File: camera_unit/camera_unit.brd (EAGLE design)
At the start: 87 x 50 mm, 0 parts

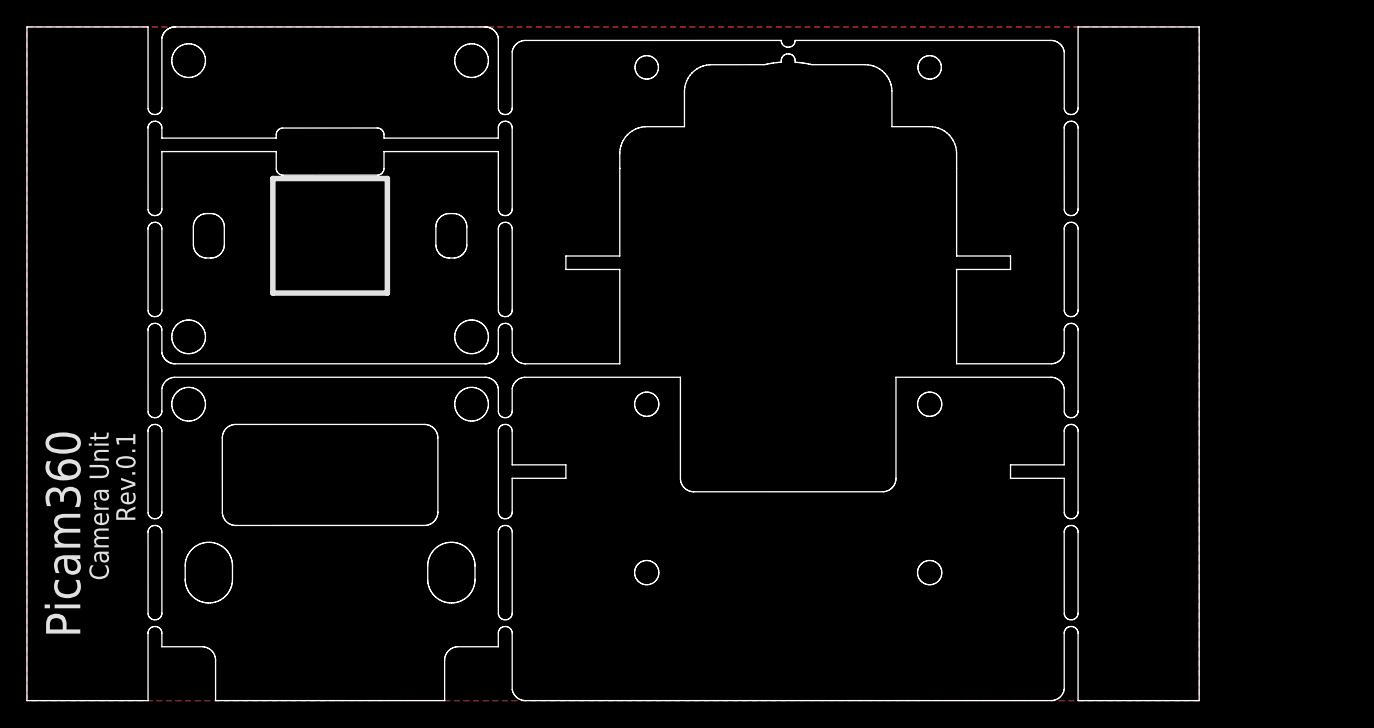
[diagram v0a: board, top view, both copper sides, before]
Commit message: before autorouter
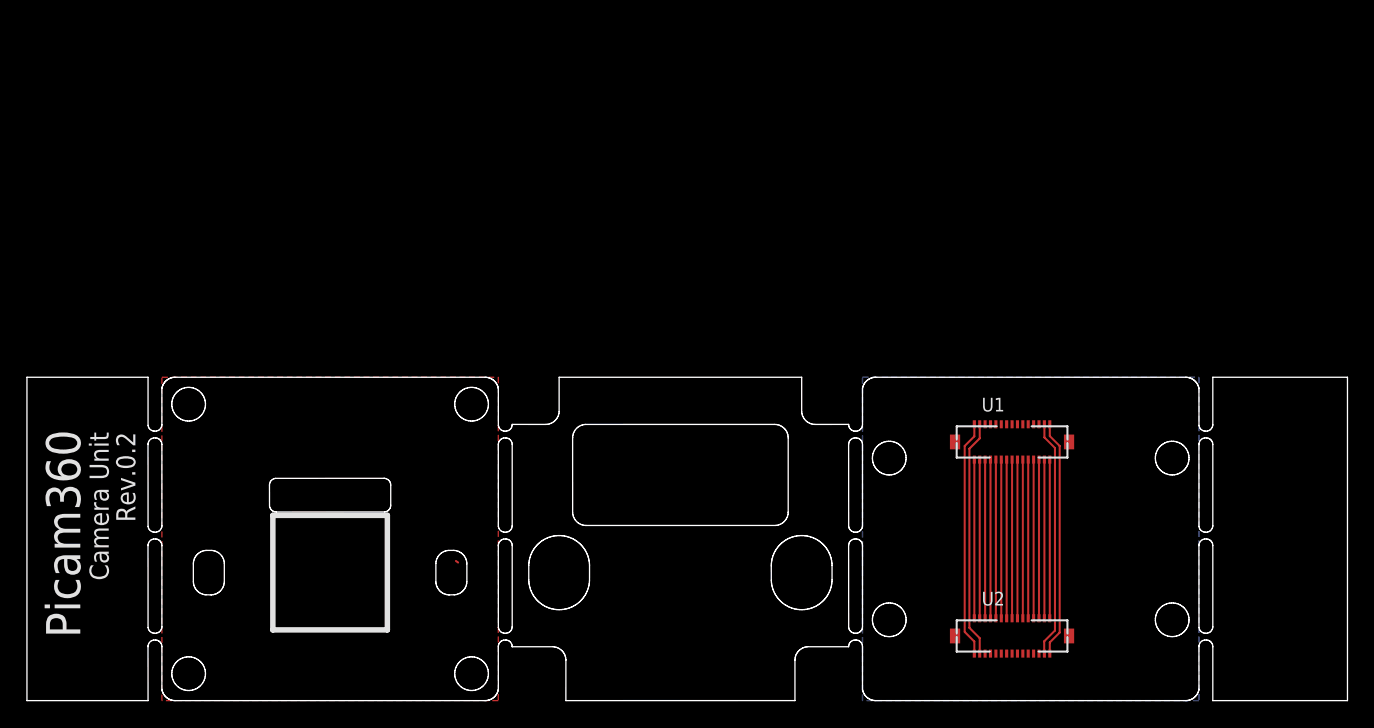
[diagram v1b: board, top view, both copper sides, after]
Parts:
- added U1: DF37*-30D*-0.4V, openblw:DF37**-30DS-0.4V
- added U2: DF37*-30D*-0.4VHEADER, openblw:DF37**-30DP-0.4V
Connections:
- new net N$1: U1.2, U2.2
- new net N$10: U1.20, U2.20
- new net N$11: U1.22, U2.22
- new net N$12: U1.24, U2.24
- new net N$13: U1.26, U2.26
- new net N$14: U1.28, U2.28
- new net N$15: U1.30, U2.30
- new net N$16: U1.1, U2.1
- new net N$17: U1.3, U2.3
- new net N$18: U1.5, U2.5
- new net N$19: U1.7, U2.7
- new net N$2: U1.4, U2.4
- new net N$20: U1.9, U2.9
- new net N$21: U1.11, U2.11
- new net N$22: U1.13, U2.13
- new net N$23: U1.15, U2.15
- new net N$24: U1.29, U2.29
- new net N$25: U1.27, U2.27
- new net N$26: U1.25, U2.25
- new net N$27: U1.23, U2.23
- new net N$28: U1.21, U2.21
- new net N$29: U1.19, U2.19
- new net N$3: U1.6, U2.6
- new net N$30: U1.17, U2.17
- new net N$4: U1.8, U2.8
- new net N$5: U1.10, U2.10
- new net N$6: U1.12, U2.12
- new net N$7: U1.14, U2.14
- new net N$8: U1.16, U2.16
- new net N$9: U1.18, U2.18
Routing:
- net N$2: track 0.00 -> 17.7 mm
- net N$14: track 0.00 -> 17.7 mm
- net N$1: track 0.00 -> 17.6 mm
- net N$15: track 0.00 -> 17.6 mm
- net N$30: track 0.00 -> 11.8 mm
- net N$29: track 0.00 -> 11.8 mm
- net N$28: track 0.00 -> 11.8 mm
- net N$27: track 0.00 -> 11.8 mm
- net N$26: track 0.00 -> 11.8 mm
- net N$25: track 0.00 -> 11.8 mm
- net N$24: track 0.00 -> 11.8 mm
- net N$23: track 0.00 -> 11.8 mm
- net N$22: track 0.00 -> 11.8 mm
- net N$21: track 0.00 -> 11.8 mm
- net N$20: track 0.00 -> 11.8 mm
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- added copper zone on layer 1, net N$31
- added copper zone on layer 16, net N$31
- removed copper zone on layer 1, net GND
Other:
- board size 87 x 50 mm -> 98 x 24 mm
- board text added: "Rev.0.2"
- board text removed: "Rev.0.1"
